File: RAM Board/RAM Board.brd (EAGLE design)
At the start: 2 parts

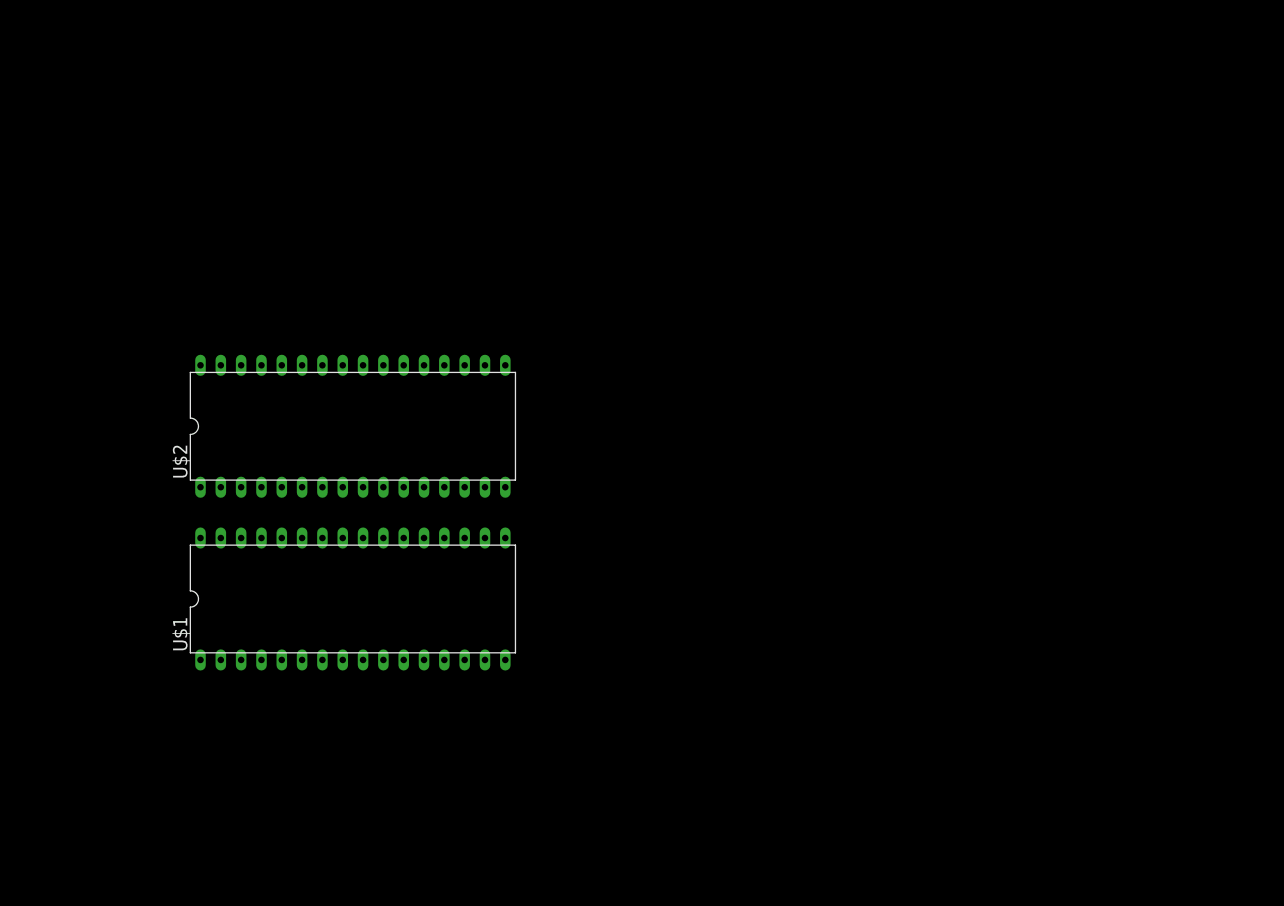
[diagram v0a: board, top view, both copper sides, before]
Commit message: Fixed more crap
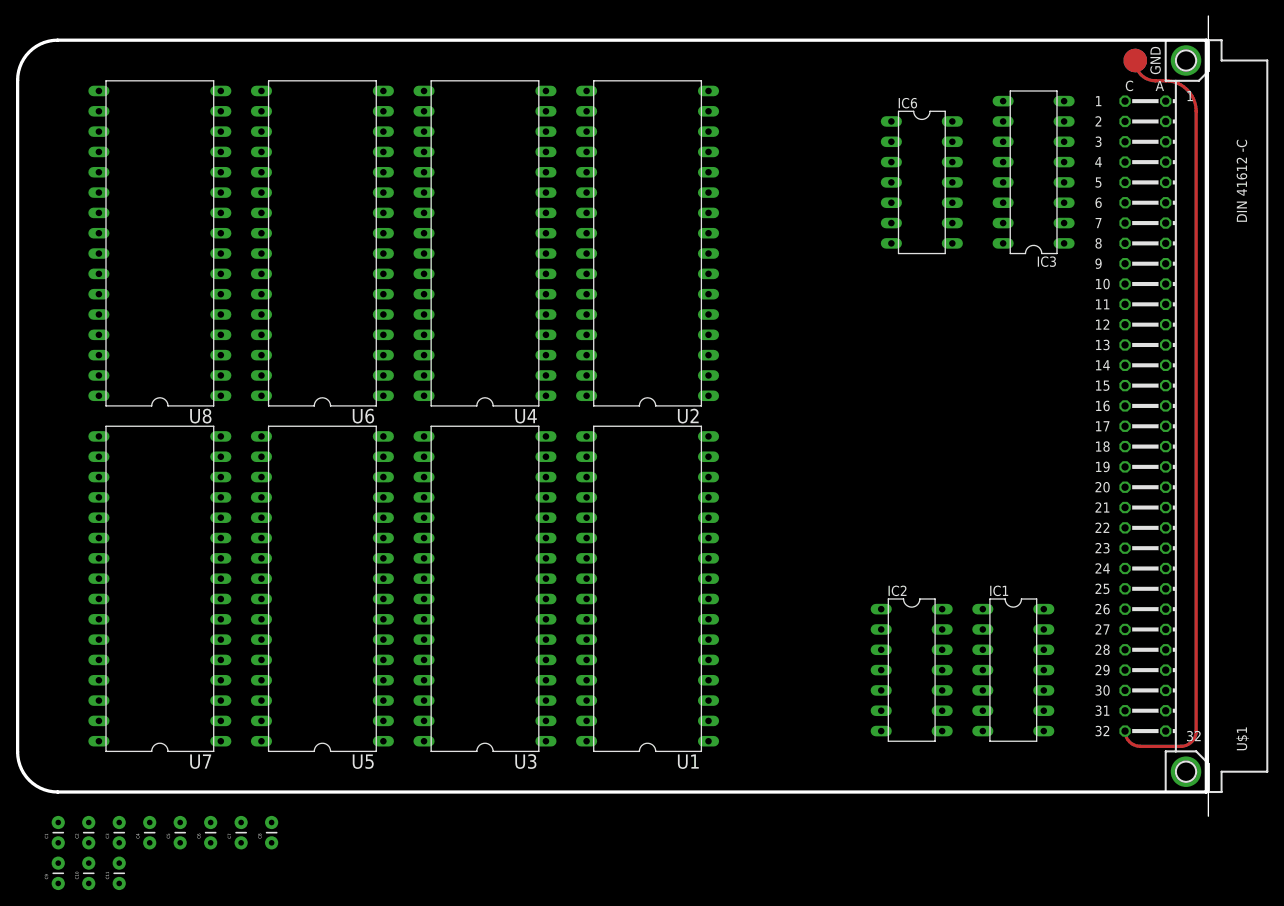
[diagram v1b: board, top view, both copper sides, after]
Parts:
- removed U$2: AS6C4008, Benchoff:DIL32
- added C1, C10, C11, C2, C3, C4, C5, C6, C7, C8, C9: 100nF, SparkFun-Capacitors:CAP-PTH-SMALL
- added IC1, IC6: 74LS32N, 74xx-us:DIL14
- added IC2: 74LS04N, 74xx-eu:DIL14
- added IC3: 74LS138N, 74xx-eu:DIL16
- added U1, U2, U3, U4, U5, U6, U7, U8: AS6C4008, Benchoff:DIL32
- U$1: value AS6C4008 -> BLANKBOARD; device Benchoff:DIL32 -> Benchoff:BLANKBOARD
- moved U$1 35.1 mm to (63.5, 50.8)
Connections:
- new net /AS: IC3.1, U$1./AS
- new net /BOOT: IC6.1, IC6.12, IC6.4, IC6.9
- new net /LDS: IC1.12, IC1.4, U$1./LDS
- new net /UDS: IC1.1, IC1.9, U$1./UDS
- new net ADDRESS20: IC3.2, U$1.A20
- new net ADDRESS21: IC3.3, U$1.A21
- new net BANKACS: IC6.6, U1.22, U2.22
- new net BANKBCS: IC6.11, U3.22, U4.22
- new net BANKCCS: IC6.8, U5.22, U6.22
- new net BANKDCS: IC6.3, U7.22, U8.22
- new net DATA11: U$1.D11, U1.17, U3.17, U5.17, U7.17
- new net N$18: IC3.9, IC6.2
- new net N$20: IC3.11, IC6.10
- new net N$22: IC3.13, IC6.13
- new net N$24: IC3.15, IC6.5
- new net N$3: IC1.2, IC1.5, IC2.2
- new net R/W: IC1.10, IC1.13, IC2.1, U$1.R/W
- new net READHI: IC1.3, U1.24, U3.24, U5.24, U7.24
- new net READLO: IC1.6, U2.24, U4.24, U6.24, U8.24
- new net WRITEHI: IC1.8, U1.29, U3.29, U5.29, U7.29
- new net WRITELO: IC1.11, U2.29, U4.29, U6.29, U8.29
- net ADDRESS0: now also U$1.A0, U1.12, U2.12, U3.12, U4.12, U5.12, U6.12, U7.12, U8.12; no longer U$1.12, U$2.12
- net ADDRESS1: now also U$1.A1, U1.11, U2.11, U3.11, U4.11, U5.11, U6.11, U7.11, U8.11; no longer U$1.11, U$2.11
- net ADDRESS10: now also U$1.A10, U1.23, U2.23, U3.23, U4.23, U5.23, U6.23, U7.23, U8.23; no longer U$1.23, U$2.23
- net ADDRESS11: now also U$1.A11, U1.25, U2.25, U3.25, U4.25, U5.25, U6.25, U7.25, U8.25; no longer U$1.25, U$2.25
- net ADDRESS12: now also U$1.A12, U1.4, U2.4, U3.4, U4.4, U5.4, U6.4, U7.4, U8.4; no longer U$1.4, U$2.4
- net ADDRESS13: now also U$1.A13, U1.28, U2.28, U3.28, U4.28, U5.28, U6.28, U7.28, U8.28; no longer U$1.28, U$2.28
- net ADDRESS14: now also U$1.A14, U1.3, U2.3, U3.3, U4.3, U5.3, U6.3, U7.3, U8.3; no longer U$1.3, U$2.3
- net ADDRESS15: now also U$1.A15, U1.31, U2.31, U3.31, U4.31, U5.31, U6.31, U7.31, U8.31; no longer U$1.31, U$2.31
- net ADDRESS16: now also U$1.A16, U1.2, U2.2, U3.2, U4.2, U5.2, U6.2, U7.2, U8.2; no longer U$1.2, U$2.2
- net ADDRESS17: now also U$1.A17, U1.30, U2.30, U3.30, U4.30, U5.30, U6.30, U7.30, U8.30; no longer U$1.30, U$2.30
- net ADDRESS18: now also U$1.A18, U1.1, U2.1, U3.1, U4.1, U5.1, U6.1, U7.1, U8.1; no longer U$1.1, U$2.1
- net ADDRESS2: now also U$1.A2, U1.10, U2.10, U3.10, U4.10, U5.10, U6.10, U7.10, U8.10; no longer U$1.10, U$2.10
- net ADDRESS3: now also U$1.A3, U1.9, U2.9, U3.9, U4.9, U5.9, U6.9, U7.9, U8.9; no longer U$1.9, U$2.9
- net ADDRESS4: now also U$1.A4, U1.8, U2.8, U3.8, U4.8, U5.8, U6.8, U7.8, U8.8; no longer U$2.8
- net ADDRESS5: now also U$1.A5, U1.7, U2.7, U3.7, U4.7, U5.7, U6.7, U7.7, U8.7; no longer U$1.7, U$2.7
- net ADDRESS6: now also U$1.A6, U1.6, U2.6, U3.6, U4.6, U5.6, U6.6, U7.6, U8.6; no longer U$1.6, U$2.6
- net ADDRESS7: now also U$1.A7, U1.5, U2.5, U3.5, U4.5, U5.5, U6.5, U7.5, U8.5; no longer U$1.5, U$2.5
- net ADDRESS8: now also U$1.A8, U1.27, U2.27, U3.27, U4.27, U5.27, U6.27, U7.27, U8.27; no longer U$1.27, U$2.27
- net ADDRESS9: now also U$1.A9, U1.26, U2.26, U3.26, U4.26, U5.26, U6.26, U7.26, U8.26; no longer U$1.26, U$2.26
- net DATA0: now also U$1.D0, U2.13, U4.13, U6.13, U8.13; no longer U$1.13
- net DATA1: now also U$1.D1, U2.14, U4.14, U6.14, U8.14; no longer U$1.14
- net DATA10: now also U$1.D10, U1.15, U3.15, U5.15, U7.15; no longer U$2.15
- net DATA12: now also U$1.D12, U1.18, U3.18, U5.18, U7.18; no longer U$2.18
- net DATA13: now also U$1.D13, U1.19, U3.19, U5.19, U7.19; no longer U$2.19
- net DATA14: now also U$1.D14, U1.20, U3.20, U5.20, U7.20; no longer U$2.20
- net DATA15: now also U$1.D15, U1.21, U3.21, U5.21, U7.21; no longer U$2.21
- net DATA2: now also U$1.D2, U2.15, U4.15, U6.15, U8.15; no longer U$1.15
- net DATA3: now also U$1.D3, U2.17, U4.17, U6.17, U8.17; no longer U$1.17
- net DATA4: now also U$1.D4, U2.18, U4.18, U6.18, U8.18; no longer U$1.18
- net DATA5: now also U$1.D5, U2.19, U4.19, U6.19, U8.19; no longer U$1.19
- net DATA6: now also U$1.D6, U2.20, U4.20, U6.20, U8.20; no longer U$1.20
- net DATA7: now also U$1.D7, U2.21, U4.21, U6.21, U8.21; no longer U$1.21
- net DATA8: now also U$1.D8, U1.13, U3.13, U5.13, U7.13; no longer U$2.13
- net DATA9: now also U$1.D9, U1.14, U3.14, U5.14, U7.14; no longer U$2.14
- net GND: now also C1.2, C10.2, C11.2, C2.2, C3.2, C4.2, C5.2, C6.2, C7.2, C8.2, C9.2, IC1.7, IC2.7, IC3.4, IC3.5, IC3.8, IC6.7, U$1.GND, U1.16, U2.16, U3.16, U4.16, U5.16, U6.16, U7.16, U8.16; no longer U$1.16, U$2.16
- net VCC: now also C1.1, C10.1, C11.1, C2.1, C3.1, C4.1, C5.1, C6.1, C7.1, C8.1, C9.1, IC1.14, IC2.14, IC3.16, IC3.6, IC6.14, U$1.5V, U1.32, U2.32, U3.32, U4.32, U5.32, U6.32, U7.32, U8.32; no longer U$1.32, U$2.32
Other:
- board outline added: 148.8 x 100 mm
